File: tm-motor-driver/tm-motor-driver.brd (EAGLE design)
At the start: 50 x 27 mm, 18 parts

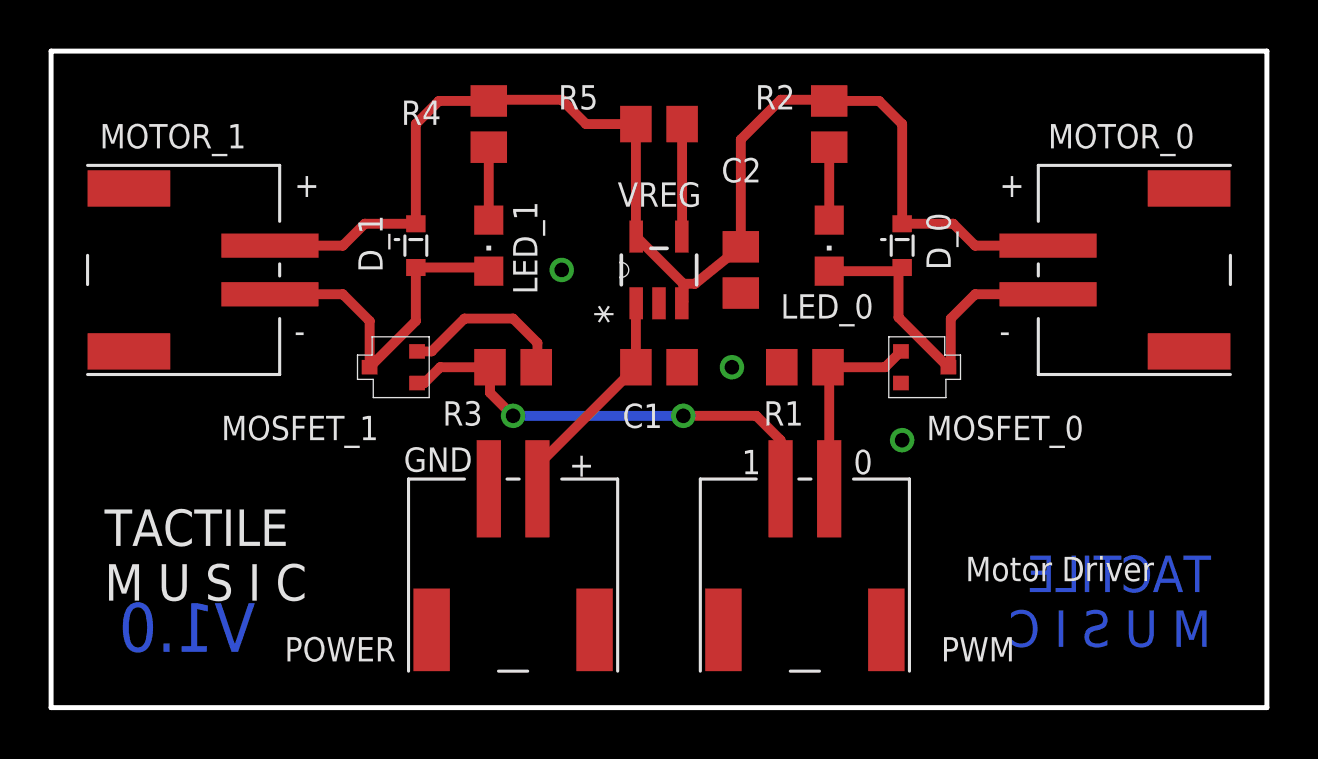
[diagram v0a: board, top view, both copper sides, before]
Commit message: Generate gerber files
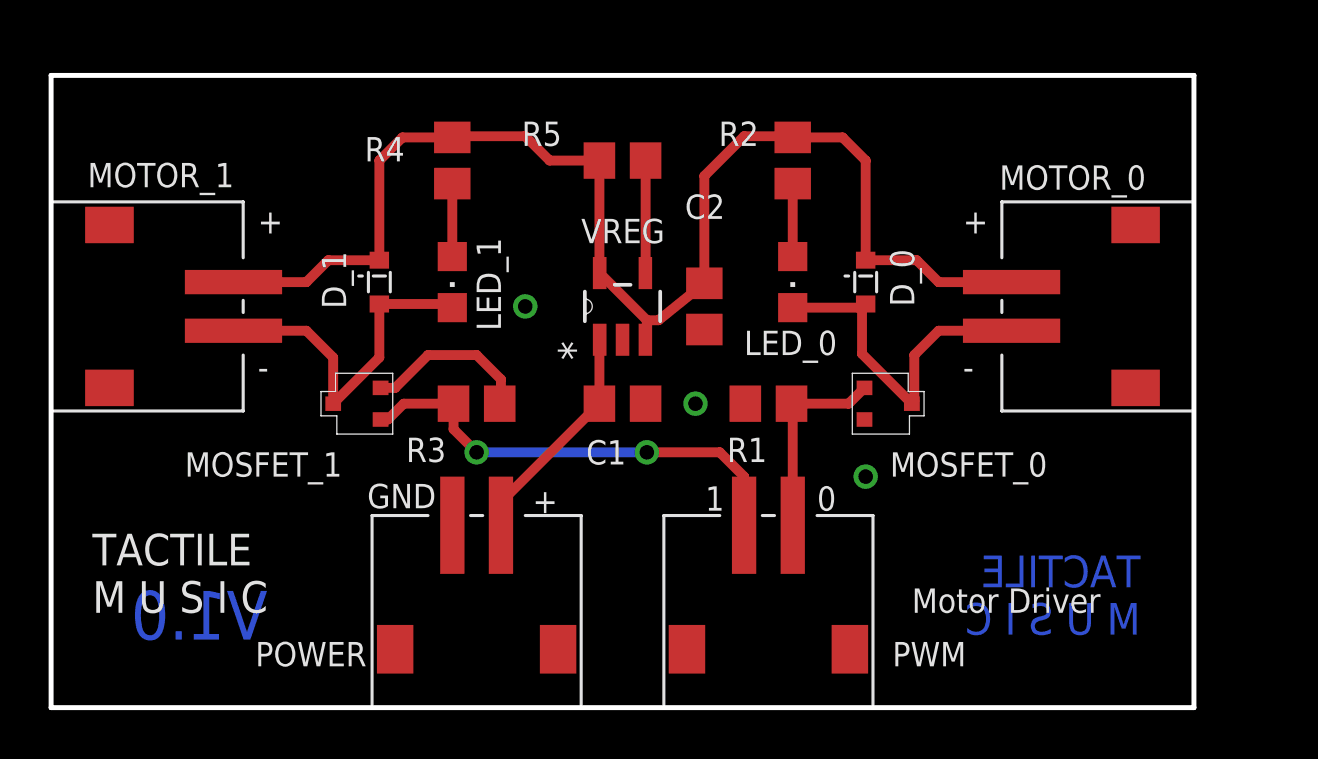
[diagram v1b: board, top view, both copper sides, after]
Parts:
- moved C1 2.12 mm to (23.5, 12.5)
- moved C2 2.12 mm to (26.9, 16.5)
- moved D_0 2.12 mm to (33.5, 17.5)
- moved D_1 2.12 mm to (13.5, 17.5)
- moved LED_0 2.12 mm to (30.5, 17.5)
- moved LED_1 2.12 mm to (16.5, 17.5)
- moved MOSFET_0 2.12 mm to (34.5, 12.5)
- moved MOSFET_1 2.12 mm to (12.5, 12.5)
- moved MOTOR_0 2.12 mm to (41.5, 16.5)
- moved MOTOR_1 2.12 mm to (5.50, 16.5)
- moved POWER 2.12 mm to (17.5, 5.50)
- moved PWM 2.12 mm to (29.5, 5.50)
- moved R1 2.12 mm to (29.5, 12.5)
- moved R2 2.12 mm to (30.5, 22.5)
- moved R3 2.12 mm to (17.5, 12.5)
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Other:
- board size 50 x 27 mm -> 47 x 26 mm
